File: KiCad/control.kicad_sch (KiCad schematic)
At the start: 7 parts, among them SW1 Encoder 1, SW2 Encoder 2, SW3 Encoder 3, SW4 Encoder 4, SW5 SW_Push, SW6 SW_Push, U11 ER_OLEDM0.91_1x-I2C

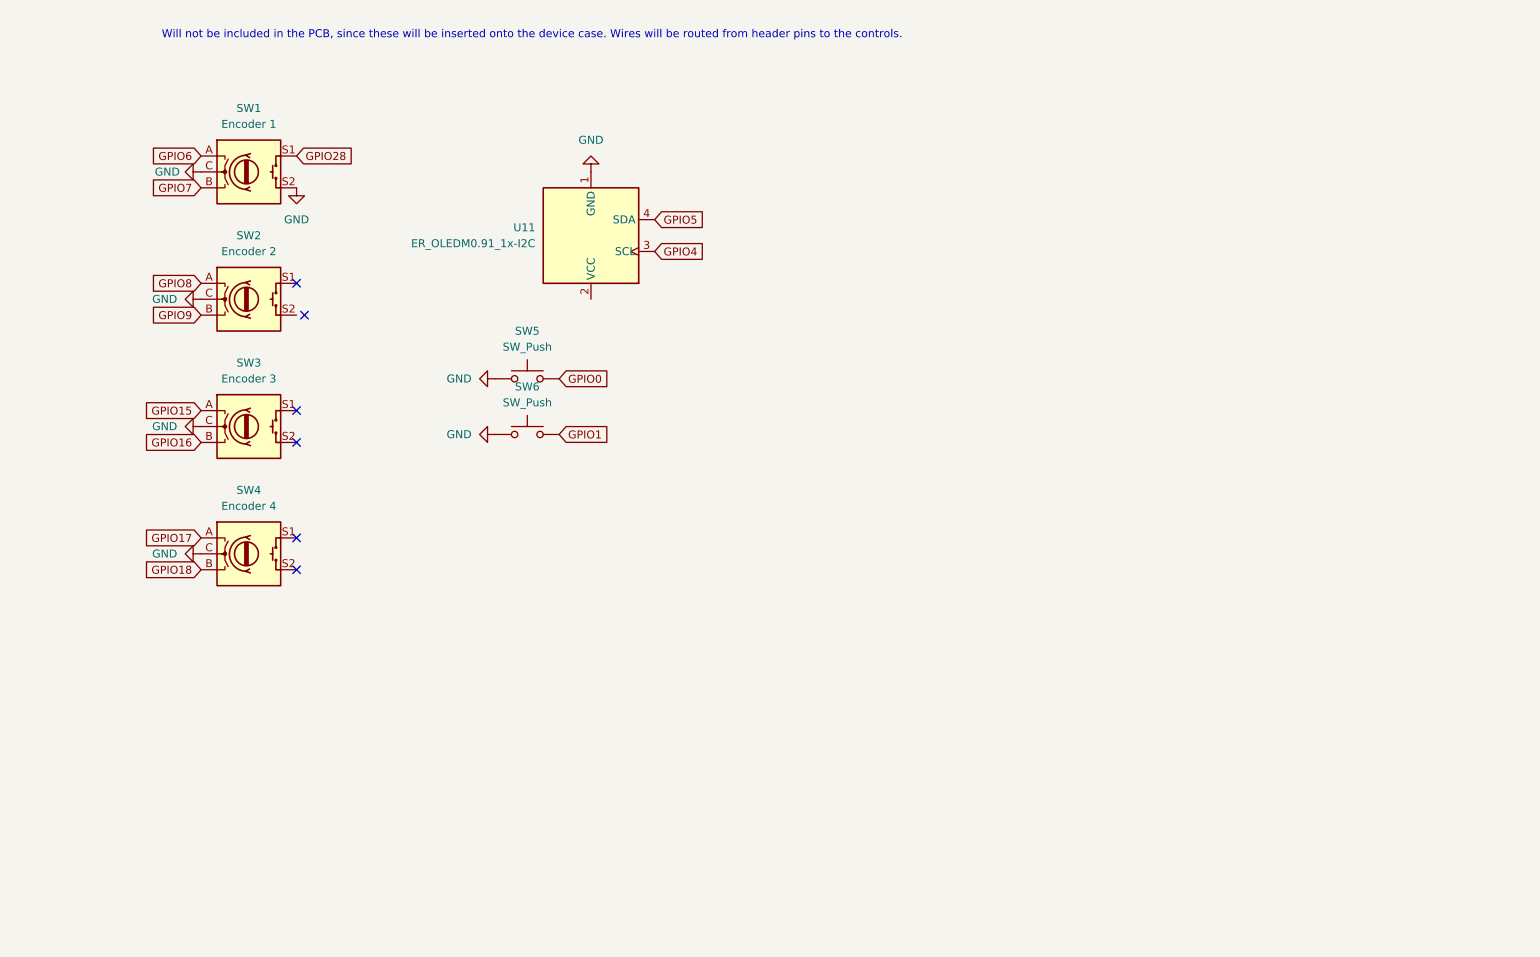
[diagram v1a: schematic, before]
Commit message: Best one yet
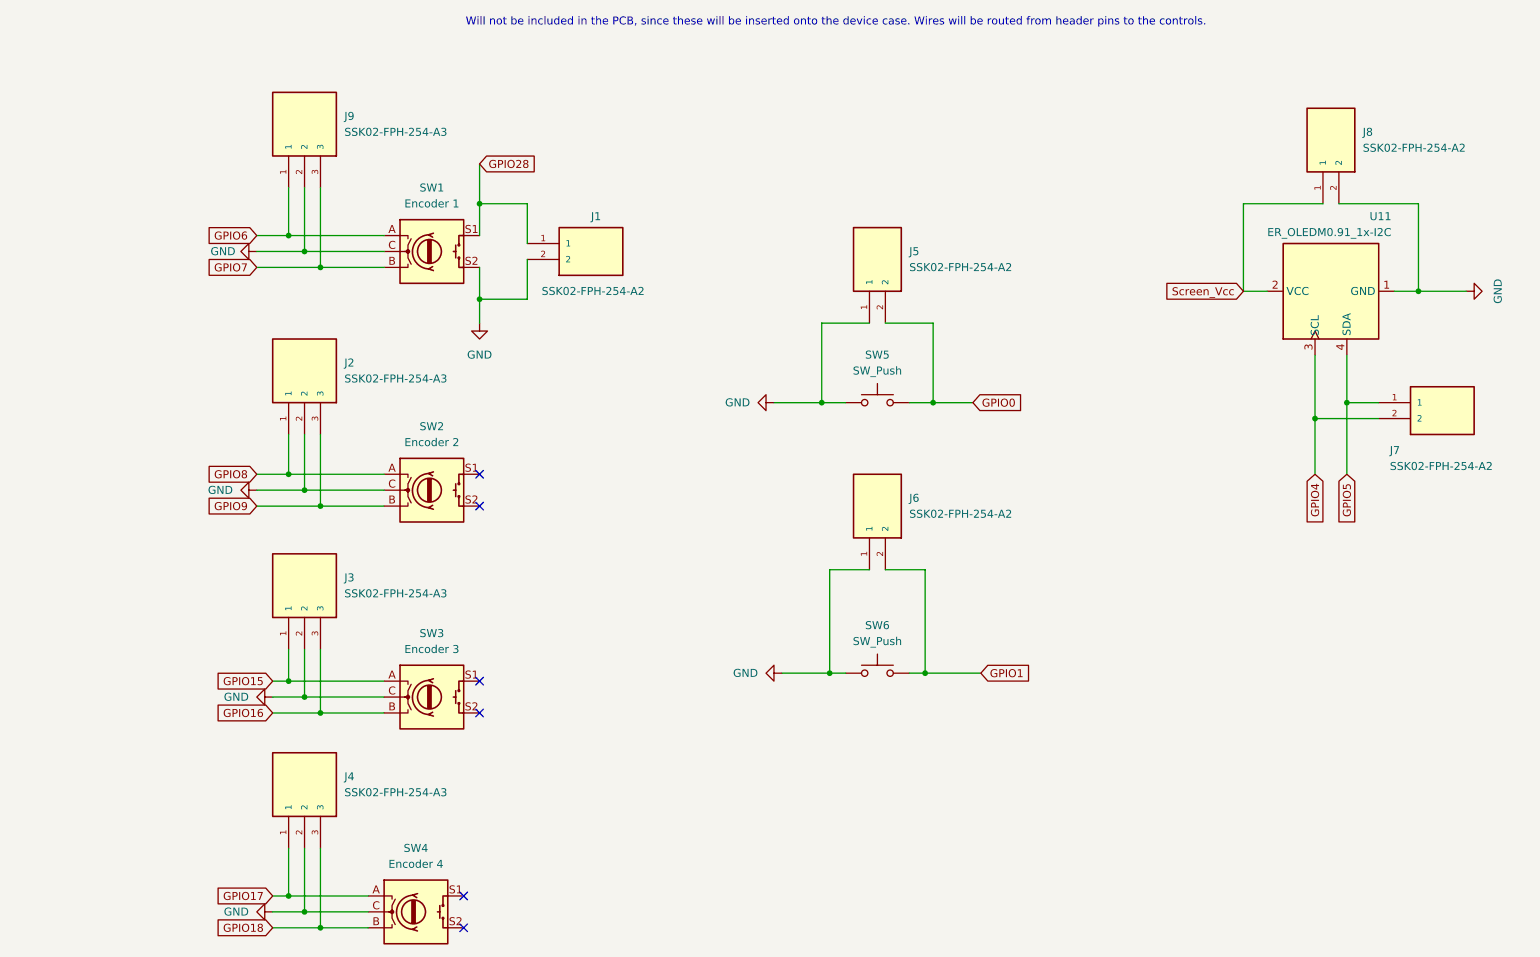
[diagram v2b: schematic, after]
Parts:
- added J1, J5, J6, J7, J8: SSK02-FPH-254-A2, SSK02-FPH-254-A2:SAMESKY_SSK02-FPH-254-A2, symbol female_headers_2pin:SSK02-FPH-254-A2
- added J2, J3, J4, J9: SSK02-FPH-254-A3, SSK02-FPH-254-A3:SAMESKY_SSK02-FPH-254-A3, symbol female_headers_3pin:SSK02-FPH-254-A3
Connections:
- net GND: now also J1.2, J2.2, J3.2, J4.2, J5.1, J6.1, J8.2, J9.2
- net GPIO0: now also J5.2
- net GPIO1: now also J6.2
- net GPIO15: now also J3.1
- net GPIO16: now also J3.3
- net GPIO17: now also J4.1
- net GPIO18: now also J4.3
- net GPIO28: now also J1.1
- net GPIO4: now also J7.2
- net GPIO5: now also J7.1
- net GPIO6: now also J9.1
- net GPIO7: now also J9.3
- net GPIO8: now also J2.1
- net GPIO9: now also J2.3
- net Screen_Vcc: now reaches U11.2 (VCC)
- net Screen_Vcc: now also J8.1
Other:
- moved on the sheet: SW1, SW2, SW3, SW4, SW5, SW6, U11
